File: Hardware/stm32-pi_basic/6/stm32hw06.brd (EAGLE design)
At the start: 54 x 55 mm, 52 parts

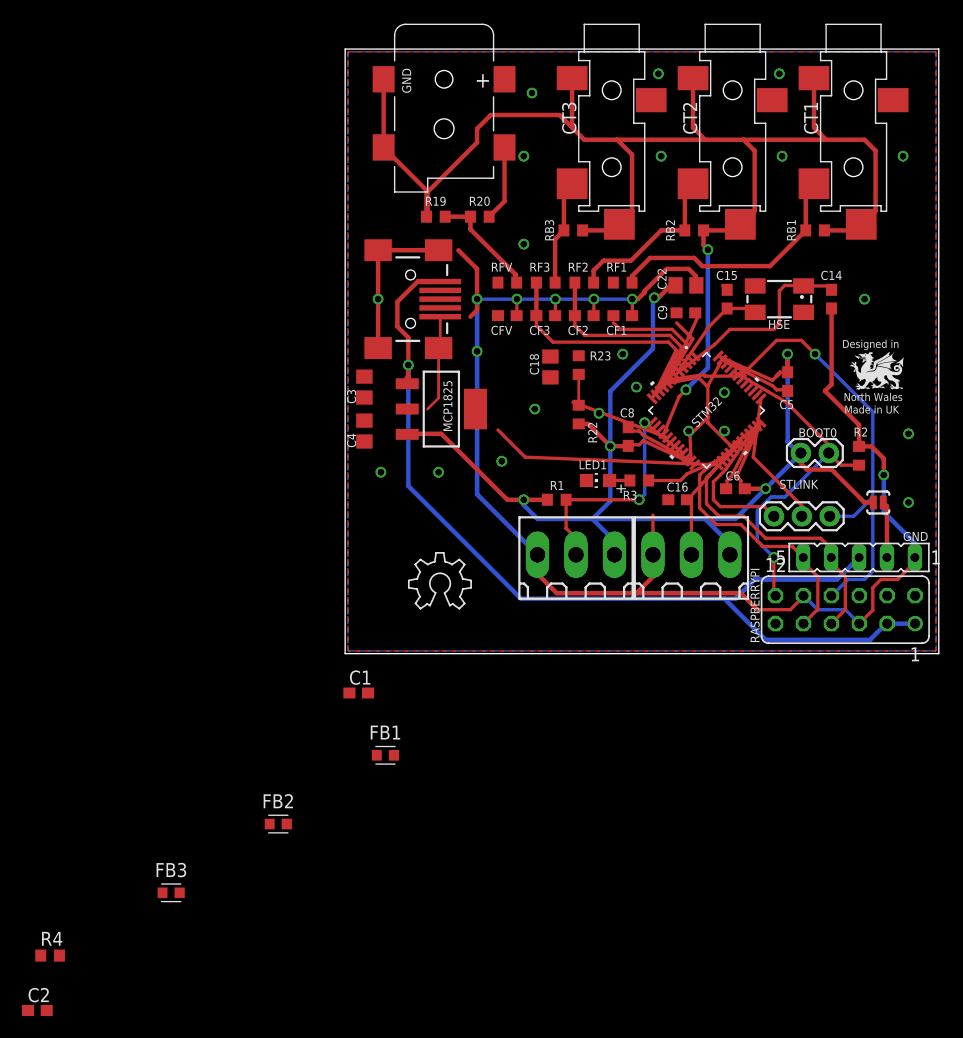
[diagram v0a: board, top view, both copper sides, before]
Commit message: modified:   Hardware/stm32-pi_basic/6/stm32hw06.brd 	modified:   Hardware/stm32-pi_full/stm32 v1.1.brd 	deleted:    Protecting Inputs in Digital Electronics ESD Protection | DigiKey.pdf
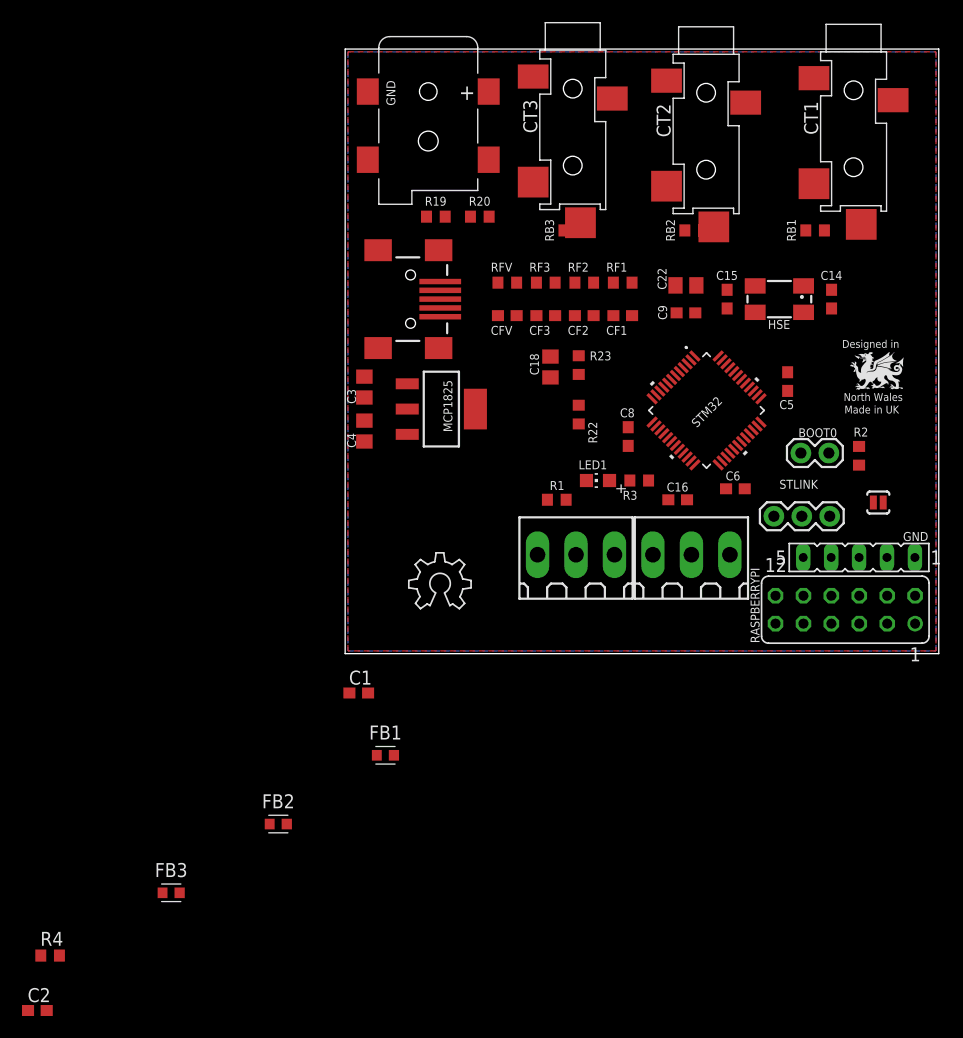
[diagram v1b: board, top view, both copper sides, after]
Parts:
- moved CT3 3.55 mm to (20.7, 54.9)
- moved CT2 2.43 mm to (32.8, 54.5)
- moved U$1 1.82 mm to (7.56, 51.1)
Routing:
- net GND: track 185.0 -> 0.00 mm, vias 28 -> 0
- net BIAS: track 142.6 -> 0.00 mm, vias 2 -> 0
- net +3V3: track 131.2 -> 0.00 mm, vias 5 -> 0
- net +5V: track 90.9 -> 0.00 mm, vias 1 -> 0
- net NRST: track 46.2 -> 0.00 mm, vias 1 -> 0
- net BOOT0: track 31.8 -> 0.00 mm, vias 1 -> 0
- net UART_RX: track 27.9 -> 0.00 mm
- net UART_TX: track 25.8 -> 0.00 mm
- net DS18B20: track 23.7 -> 0.00 mm, vias 2 -> 0
- net N$2: track 23.3 -> 0.00 mm
- net GND_USB: track 23.3 -> 0.00 mm, vias 1 -> 0
- net CT3: track 22.5 -> 0.00 mm
- net VSIG: track 21.1 -> 0.00 mm
- net CT2: track 19.4 -> 0.00 mm
- net HSE_IN: track 18.8 -> 0.00 mm
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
